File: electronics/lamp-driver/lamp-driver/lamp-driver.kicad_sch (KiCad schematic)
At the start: 30 parts, among them J1 Conn_01x04_Pin, J12V1 Conn_01x02_Pin, J2 Conn_01x04_Pin, J3 Conn_01x04_Pin, J4 Conn_01x04_Pin, J5 Conn_01x04_Pin, J6 Conn_01x04_Pin, Q1 AO3400A, U1 LM78M05_TO252

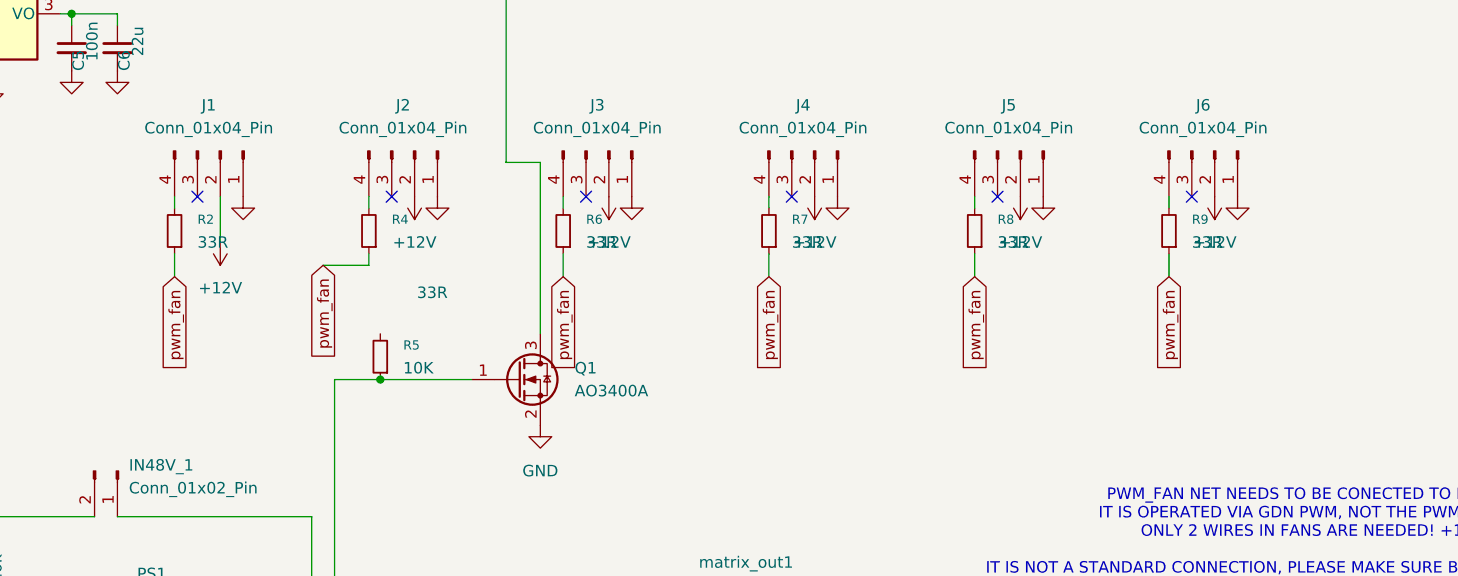
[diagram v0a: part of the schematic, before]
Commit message: uv control fixed
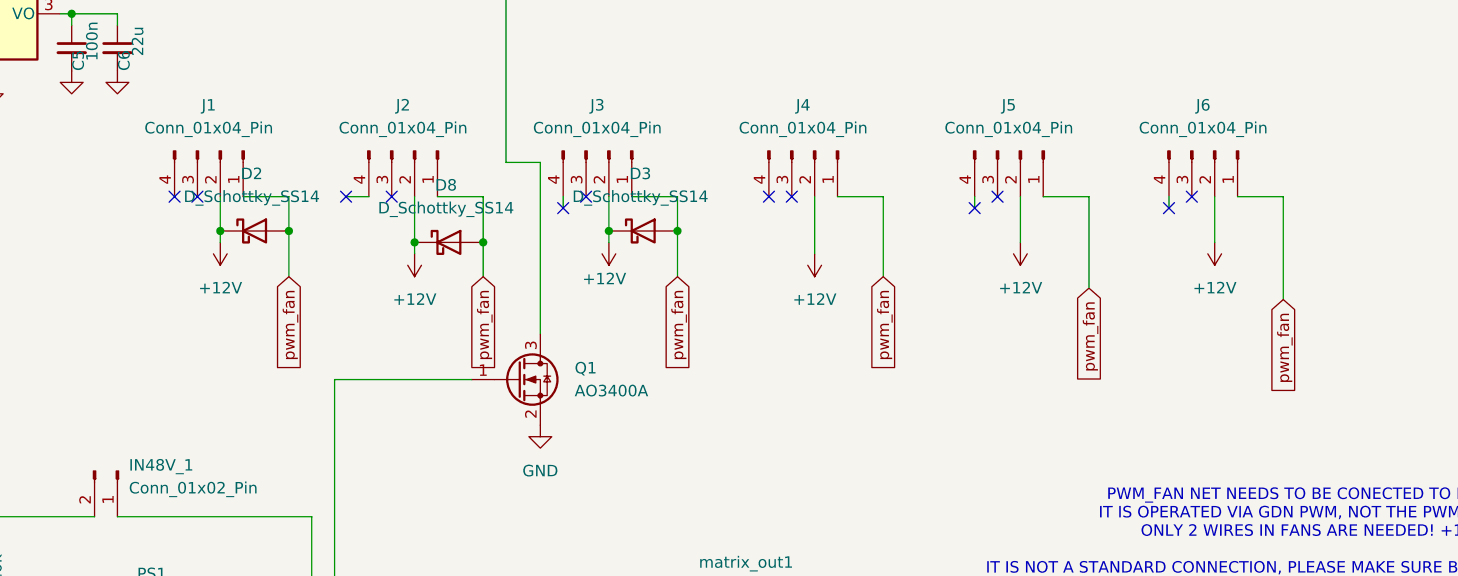
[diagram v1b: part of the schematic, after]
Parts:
- removed R2, R4, R6, R7, R8, R9: 33R, Resistor_SMD:R_0805_2012Metric, symbol Device:R_Small
- removed R5: 10K, Resistor_SMD:R_0805_2012Metric, symbol Device:R_Small
- added D2, D3, D8: D_Schottky_SS14, Diode_SMD:D_SMA, symbol Device:D_Schottky
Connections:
- net +12V: now also D2.1 (K), D3.1 (K), D8.1 (K)
- net GND: no longer J1.1 (Pin_1), J2.1 (Pin_1), J3.1 (Pin_1), J4.1 (Pin_1), J5.1 (Pin_1), J6.1 (Pin_1)
- net pwm_fan: now also J1.1 (Pin_1), J2.1 (Pin_1), J3.1 (Pin_1), J4.1 (Pin_1), J5.1 (Pin_1), J6.1 (Pin_1), D2.2 (A), D3.2 (A), D8.2 (A)
- no-connect marks 8 -> 14
